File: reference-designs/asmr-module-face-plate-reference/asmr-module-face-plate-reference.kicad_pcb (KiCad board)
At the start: 2 copper layers, 40 x 159.8 mm, 0 parts

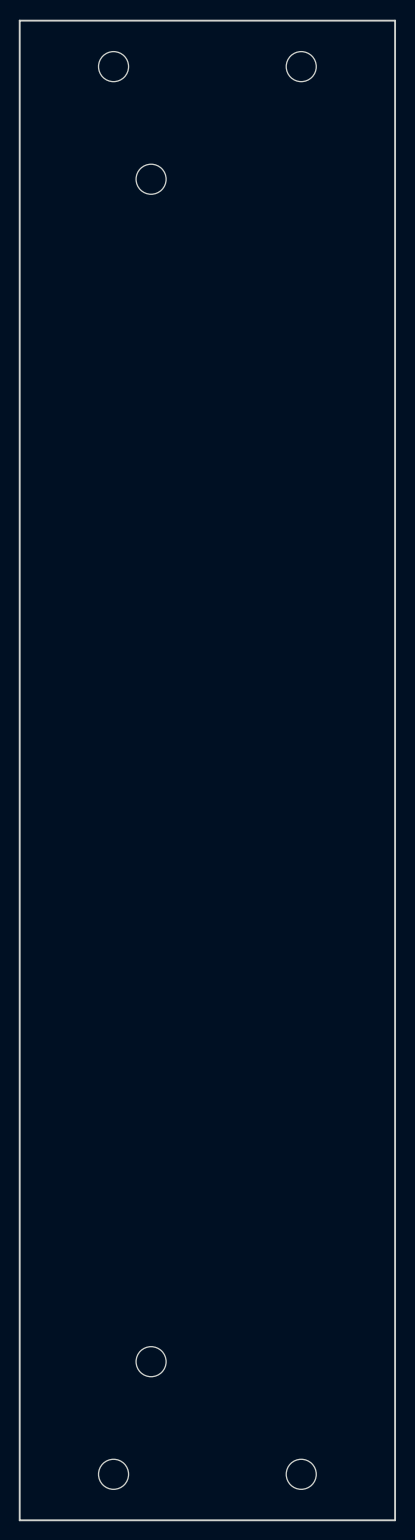
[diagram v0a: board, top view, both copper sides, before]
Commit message: Tune faceplate design.
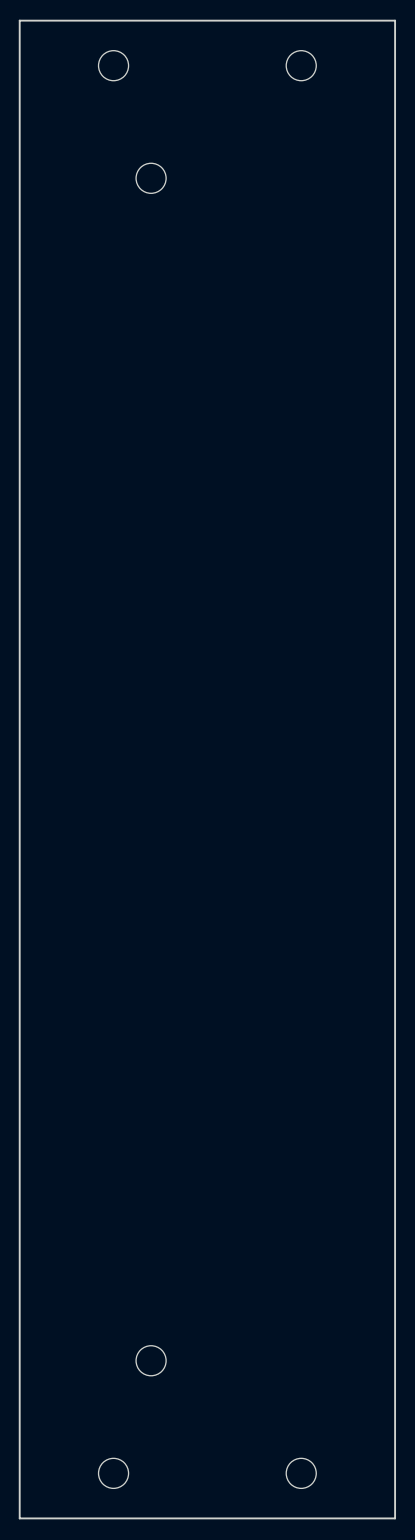
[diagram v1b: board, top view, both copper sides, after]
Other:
- board size 40 x 159.8 mm -> 40 x 159.6 mm
- board text added: "A S M R"
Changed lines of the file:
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@@
 	(net 0 "")
 	(gr_circle
-		(center 104 67.1)
-		(end 105.6 67.1)
+		(center 104 67)
+		(end 105.6 67)
+		(stroke
+			(width 0.1)
+			(type default)
+		)
+		(fill no)
+		(layer "Dwgs.User")
+	)
+	(gr_circle
+		(center 100 55)
+		(end 103 55)
 		(stroke
 			(width 0.1)
@@
 	)
 	(gr_line
-		(start 90 60.1)
-		(end 130 60.1)
+		(start 90 60)
+		(end 130 60)
 		(stroke
 			(width 0.3)
@@
 		(layer "Dwgs.User")
 	)
-	(gr_rect
-		(start 99 188.1)
-		(end 109.2 198.1)
+	(gr_circle
+		(center 120 55)
+		(end 123 55)
+		(stroke
+			(width 0.1)
+			(type default)
+		)
+		(fill no)
+		(layer "Dwgs.User")
+	)
+	(gr_rect
+		(start 99 188)
+		(end 109.2 198)
 		(stroke
 			(width 0.1)
@@
 	)
 	(gr_circle
-		(center 104 193.1)
-		(end 105.6 193.1)
+		(center 104 193)
+		(end 105.6 193)
+		(stroke
+			(width 0.1)
+			(type default)
+		)
+		(fill no)
+		(layer "Dwgs.User")
+	)
+	(gr_circle
+		(center 100 205)
+		(end 103 205)
 		(stroke
 			(width 0.1)
@@
 	)
 	(gr_line
-		(start 90 200.1)
+		(start 90 200)
 		(end 130 200.1)
 		(stroke
@@
 		(layer "Dwgs.User")
 	)
-	(gr_rect
-		(start 99 62.1)
-		(end 109.2 72.1)
-		(stroke
-			(width 0.1)
-			(type default)
-		)
-		(fill no)
-		(layer "Dwgs.User")
-	)
-	(gr_rect
-		(start 109.2 62.1)
-		(end 110.8 198.1)
+	(gr_circle
+		(center 120 205)
+		(end 123 205)
+		(stroke
+			(width 0.1)
+			(type default)
+		)
+		(fill no)
+		(layer "Dwgs.User")
+	)
+	(gr_rect
+		(start 99 62)
+		(end 109.2 72)
+		(stroke
+			(width 0.1)
+			(type default)
+		)
+		(fill no)
+		(layer "Dwgs.User")
+	)
+	(gr_rect
+		(start 109.2 62)
+		(end 110.8 198)
 		(stroke
 			(width 0.1)
@@
 	(gr_rect
 		(start 90 50.2)
-		(end 130 210)
+		(end 130 209.8)
 		(stroke
 			(width 0.2)
@@
 	)
 	(gr_circle
-		(center 104 193.1)
-		(end 105.6 193.1)
-		(stroke
-			(width 0.05)
-			(type default)
-		)
-		(fill no)
-		(layer "Edge.Cuts")
-	)
-	(gr_circle
-		(center 120 205.1)
-		(end 121.6 205.1)
-		(stroke
-			(width 0.05)
-			(type default)
-		)
-		(fill no)
-		(layer "Edge.Cuts")
-	)
-	(gr_circle
-		(center 100 205.1)
-		(end 101.6 205.1)
-		(stroke
-			(width 0.05)
-			(type default)
-		)
-		(fill no)
-		(layer "Edge.Cuts")
-	)
-	(gr_circle
-		(center 104 67.1)
-		(end 105.6 67.1)
-		(stroke
-			(width 0.05)
-			(type default)
-		)
-		(fill no)
-		(layer "Edge.Cuts")
-	)
-	(gr_circle
-		(center 120 55.1)
-		(end 121.6 55.1)
-		(stroke
-			(width 0.05)
-			(type default)
-		)
-		(fill no)
-		(layer "Edge.Cuts")
-	)
-	(gr_circle
-		(center 100 55.1)
-		(end 101.6 55.1)
-		(stroke
-			(width 0.05)
-			(type default)
-		)
-		(fill no)
-		(layer "Edge.Cuts")
+		(center 104 193)
+		(end 105.6 193)
+		(stroke
+			(width 0.05)
+			(type default)
+		)
+		(fill no)
+		(layer "Edge.Cuts")
+	)
+	(gr_circle
+		(center 120 205)
+		(end 121.6 205)
+		(stroke
+			(width 0.05)
+			(type default)
+		)
+		(fill no)
+		(layer "Edge.Cuts")
+	)
+	(gr_circle
+		(center 100 205)
+		(end 101.6 205)
+		(stroke
+			(width 0.05)
+			(type default)
+		)
+		(fill no)
+		(layer "Edge.Cuts")
+	)
+	(gr_circle
+		(center 104 67)
+		(end 105.6 67)
+		(stroke
+			(width 0.05)
+			(type default)
+		)
+		(fill no)
+		(layer "Edge.Cuts")
+	)
+	(gr_circle
+		(center 120 55)
+		(end 121.6 55)
+		(stroke
+			(width 0.05)
+			(type default)
+		)
+		(fill no)
+		(layer "Edge.Cuts")
+	)
+	(gr_circle
+		(center 100 55)
+		(end 101.6 55)
+		(stroke
+			(width 0.05)
+			(type default)
+		)
+		(fill no)
+		(layer "Edge.Cuts")
+	)
+	(gr_rect
+		(start 90 198.5)
+		(end 130 209.8)
+		(stroke
+			(width 0.05)
+			(type default)
+		)
+		(fill no)
+		(layer "B.CrtYd")
+	)
+	(gr_rect
+		(start 90 50)
+		(end 130 61.5)
+		(stroke
+			(width 0.05)
+			(type default)
+		)
+		(fill no)
+		(layer "B.CrtYd")
+	)
+	(gr_text "A      S      M      R"
+		(at 110 52.5 0)
+		(layer "F.Mask")
+		(effects
+			(font
+				(face "Audiowide")
+				(size 2.3 2.5)
+				(thickness 0.4)
+				(bold yes)
+			)
+		)
+		(render_cache "A      S      M      R" 0
+			(polygon
+				(pts
+					(xy 96.343619 51.208589) (xy 96.416892 51.25353) (xy 96.465741 51.321081) (xy 96.483296 51.402817)
+					(xy 96.483296 53.4545) (xy 96.029462 53.4545) (xy 96.029462 52.901448) (xy 94.478367 52.901448)
+					(xy 94.478367 53.4545) (xy 94.024534 53.4545) (xy 94.024534 52.323539) (xy 94.478367 52.323539)
+					(xy 94.478367 52.483921) (xy 96.029462 52.483921) (xy 96.029462 51.609965) (xy 95.253991 51.609965)
+					(xy 95.168201 51.615442) (xy 95.017075 51.642828) (xy 94.931135 51.669689) (xy 94.836183 51.709958)
+					(xy 94.746062 51.763026) (xy 94.661549 51.834669) (xy 94.590285 51.922) (xy 94.530116 52.033672)
+					(xy 94.492269 52.160537) (xy 94.478367 52.323539) (xy 94.024534 52.323539) (xy 94.035183 52.160195)
+					(xy 94.066307 52.008842) (xy 94.117193 51.867812) (xy 94.187761 51.734153) (xy 94.273394 51.615241)
+					(xy 94.374411 51.509691) (xy 94.49016 51.417569) (xy 94.619455 51.339832) (xy 94.763673 51.27614)
+					(xy 94.915869 51.230145) (xy 95.078733 51.202043) (xy 95.253991 51.192438) (xy 96.254776 51.192438)
+				)
+			)
+			(polygon
+				(pts
+					(xy 106.181569 52.78699) (xy 106.172798 52.904952) (xy 106.147985 53.005935) (xy 106.108336 53.098753)
+					(xy 106.059295 53.177553) (xy 105.999203 53.246798) (xy 105.930304 53.304229) (xy 105.854479 53.352092)
+					(xy 105.777347 53.389757) (xy 105.616604 53.43877) (xy 105.462731 53.4545) (xy 103.744941 53.4545)
+					(xy 103.744941 53.036972) (xy 105.462731 53.036972) (xy 105.543578 53.028767) (xy 105.607414 53.005921)
+					(xy 105.658126 52.969281) (xy 105.695867 52.920534) (xy 105.719358 52.86079) (xy 105.727735 52.78699)
+					(xy 105.722977 52.732821) (xy 105.709264 52.68489) (xy 105.686618 52.641358) (xy 105.656446 52.604699)
+					(xy 105.618625 52.57487) (xy 105.572641 52.552315) (xy 105.521386 52.538561) (xy 105.462731 52.533777)
+					(xy 104.441491 52.533777) (xy 104.331687 52.525323) (xy 104.207628 52.498246) (xy 104.087446 52.452165)
+					(xy 103.974834 52.383647) (xy 103.87779 52.293856) (xy 103.795927 52.176358) (xy 103.757528 52.088513)
+					(xy 103.733148 51.985107) (xy 103.724486 51.863178) (xy 103.733164 51.741245) (xy 103.757558 51.638145)
+					(xy 103.795927 51.55084) (xy 103.877719 51.433706) (xy 103.974834 51.343551) (xy 104.087505 51.27437)
+					(xy 104.207628 51.22811) (xy 104.331692 51.200925) (xy 104.441491 51.192438) (xy 105.957781 51.192438)
+					(xy 105.957781 51.609965) (xy 104.441491 51.609965) (xy 104.361923 51.618303) (xy 104.298592 51.641639)
+					(xy 104.247776 51.679342) (xy 104.210073 51.728945) (xy 104.186649 51.789245) (xy 104.178319 51.863178)
+					(xy 104.186739 51.938016) (xy 104.210232 51.997921) (xy 104.247776 52.046171) (xy 104.298391 52.082472)
+					(xy 104.361717 52.105064) (xy 104.441491 52.113161) (xy 105.462731 52.113161) (xy 105.466242 52.113161)
+					(xy 105.619199 52.131418) (xy 105.779942 52.182819) (xy 105.85758 52.221873) (xy 105.932136 52.270593)
+					(xy 105.999769 52.328426) (xy 106.06021 52.397972) (xy 106.109794 52.476762) (xy 106.148901 52.568887)
+					(xy 106.173007 52.668985)
+				)
+			)
+			(polygon
+				(pts
+					(xy 116.213691 53.4545) (xy 115.756499 53.4545) (xy 115.756499 52.125238) (xy 114.978433 53.384701)
+					(xy 114.942647 53.428647) (xy 114.89539 53.460258) (xy 114.840293 53.479513) (xy 114.781207 53.485958)
+					(xy 114.72369 53.479514) (xy 114.670229 53.460258) (xy 114.624386 53.428758) (xy 114.589018 53.384701)
+					(xy 113.807441 52.125238) (xy 113.807441 53.4545) (xy 113.353607 53.4545) (xy 113.353607 51.371358)
+					(xy 113.365246 51.30286) (xy 113.399861 51.242856) (xy 113.453193 51.195998) (xy 113.521219 51.16744)
+					(xy 113.594492 51.161822) (xy 113.665169 51.176288) (xy 113.727146 51.210134) (xy 113.774468 51.262237)
+					(xy 114.781207 52.872237) (xy 115.787945 51.262237) (xy 115.83587 51.20988) (xy 115.89877 51.175445)
+					(xy 115.970579 51.160613) (xy 116.046079 51.16744) (xy 116.112832 51.19587) (xy 116.166521 51.242856)
+					(xy 116.201843 51.302918) (xy 116.213691 51.371358)
+				)
+			)
+			(polygon
+				(pts
+					(xy 126.007829 51.954183) (xy 125.997896 52.09035) (xy 125.969971 52.205429) (xy 125.924835 52.310855)
+					(xy 125.867695 52.40064) (xy 125.797863 52.479551) (xy 125.719012 52.545434) (xy 125.6324 52.600516)
+					(xy 125.543004 52.644303) (xy 125.450053 52.677814) (xy 125.357532 52.700339) (xy 125.194653 52.717613)
+					(xy 126.122013 53.4545) (xy 125.420425 53.4545) (xy 124.494897 52.717613) (xy 124.172497 52.717613)
+					(xy 124.172497 52.300086) (xy 125.181372 52.300086) (xy 125.261483 52.288834) (xy 125.332345 52.268346)
+					(xy 125.396597 52.23793) (xy 125.450345 52.19939) (xy 125.494171 52.151827) (xy 125.526976 52.094763)
+					(xy 125.546926 52.030615) (xy 125.553995 51.954183) (xy 125.553995 51.696617) (xy 125.545142 51.646058)
+					(xy 125.522854 51.62092) (xy 125.493851 51.61151) (xy 125.464999 51.609965) (xy 124.00458 51.609965)
+					(xy 124.00458 53.4545) (xy 123.550746 53.4545) (xy 123.550746 51.402817) (xy 123.568148 51.321081)
+					(xy 123.616234 51.25353) (xy 123.688743 51.208589) (xy 123.779418 51.192438) (xy 125.464999 51.192438)
+					(xy 125.607176 51.20574) (xy 125.718249 51.242435) (xy 125.813189 51.299665) (xy 125.886318 51.367847)
+					(xy 125.942266 51.446608) (xy 125.979436 51.530196) (xy 126.001047 51.616366) (xy 126.007829 51.693386)
+				)
+			)
+		)
 	)
 	(gr_text "Chassis Rail"
-		(at 110 60.1 0)
+		(at 110 59.6 0)
 		(layer "Cmts.User")
 		(effects

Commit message: Tune deisgn.
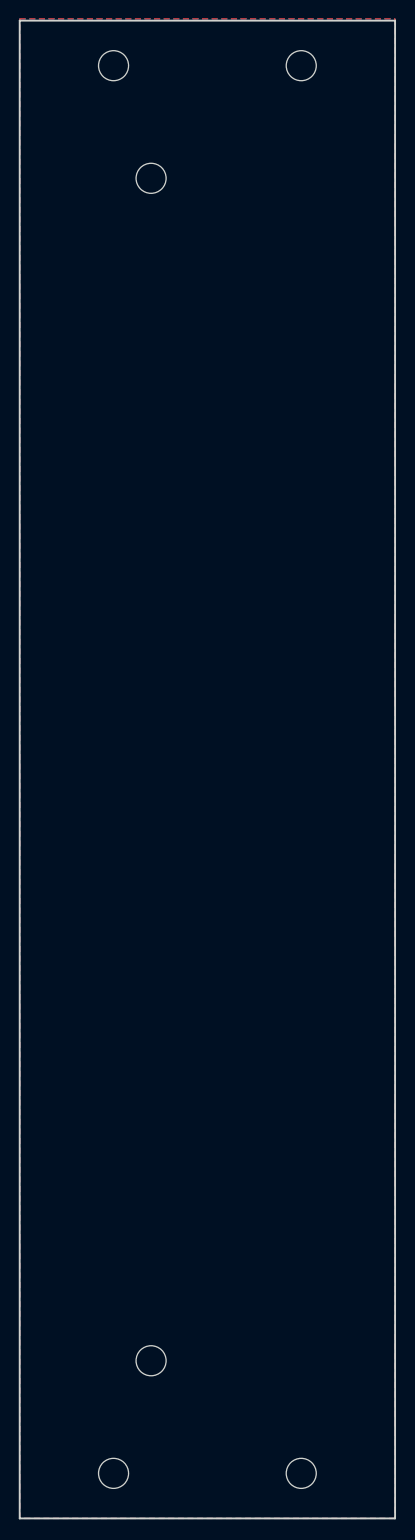
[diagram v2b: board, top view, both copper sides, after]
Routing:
- added copper zone on B.Cu, net (none)
- added copper zone on F.Cu, net (none)
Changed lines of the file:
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@@
+		)
+	)
+	(zone
+		(net 0)
+		(net_name "")
+		(layers "F.Cu" "B.Cu")
+		(hatch edge 0.5)
+		(connect_pads
+			(clearance 0.3)
+		)
+		(min_thickness 0.2)
+		(filled_areas_thickness no)
+		(fill yes
+			(thermal_gap 0.5)
+			(thermal_bridge_width 0.5)
+			(island_removal_mode 1)
+			(island_area_min 10)
+		)
+		(polygon
+			(pts
+				(xy 90 50) (xy 130 50) (xy 130 209.8) (xy 90 209.8)
+			)
 		)
 	)
